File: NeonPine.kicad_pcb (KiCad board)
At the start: 2 copper layers, 54.7 x 69 mm, 102 parts, among them J1 USB-C 16P (USB4105-GF-A), J2 SWD pogo pads, Q1 DMN15H310SE, Q11 MMDT5551, Q12 MMDT5551, Q13 MMDT5551, Q14 MMDT5551, Q15 MMDT5551, Q16 MMDT5551, Q17 MMDT5551, Q18 MMDT5551, Q19 MMDT5551, Q2 TEPT4400, Q20 MMDT5551, U1 CH32V003F4P6, U2 74HC595BQ, U3 74HC595BQ

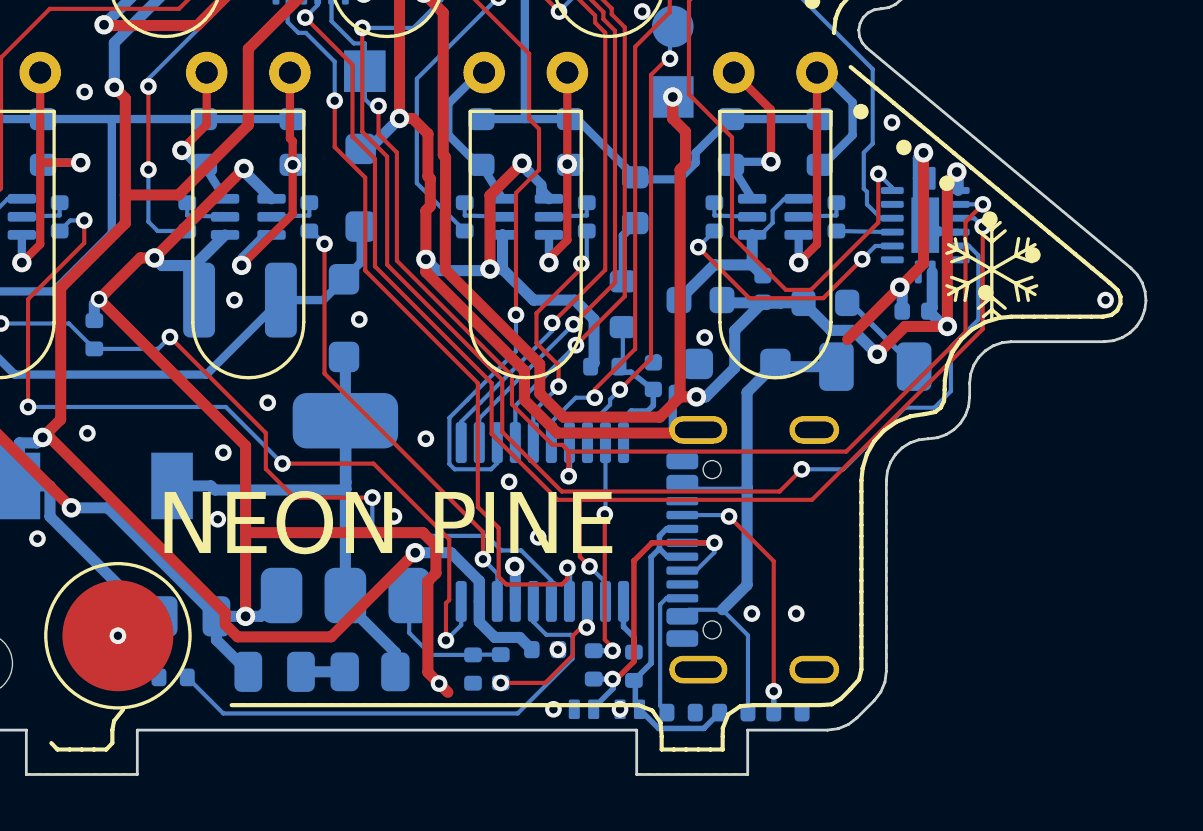
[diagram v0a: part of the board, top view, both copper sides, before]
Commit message: USB clearance fix
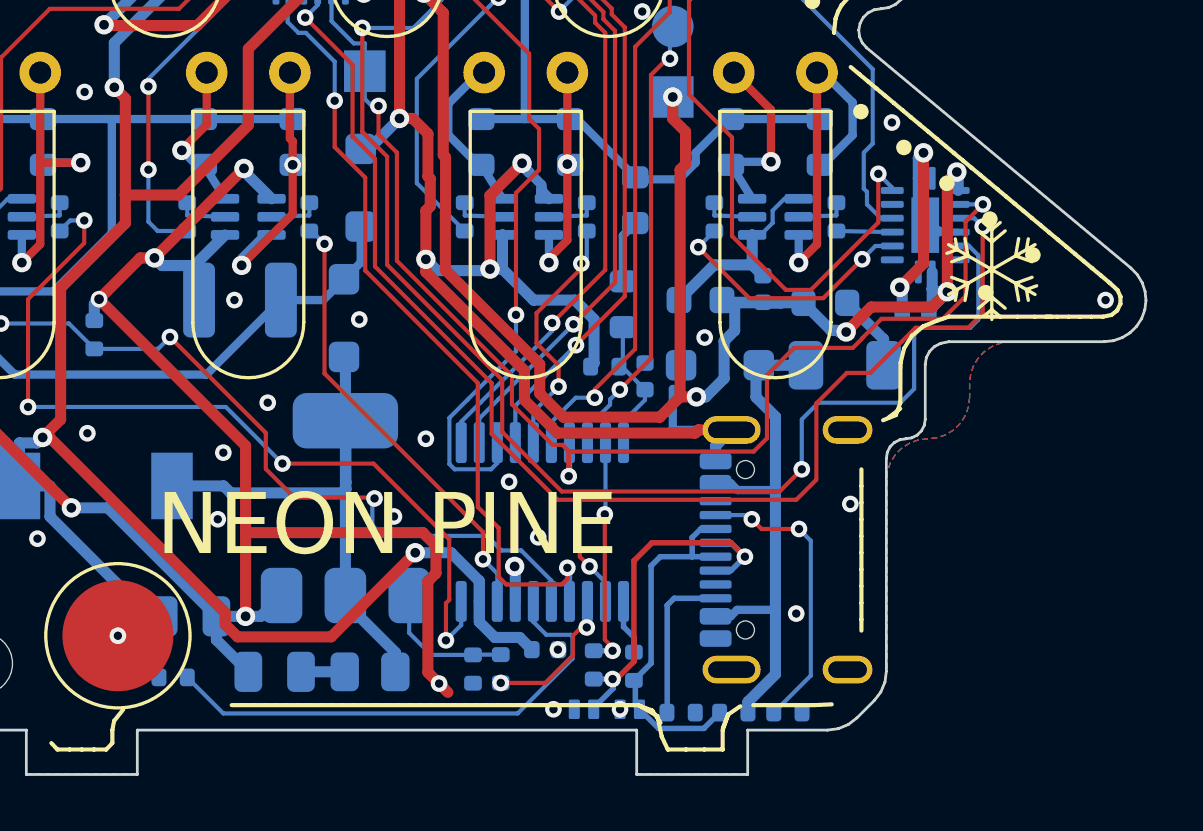
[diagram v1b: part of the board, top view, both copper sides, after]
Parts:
- moved J1 1.20 mm to (115.5, 103.5)
- moved F1 1.10 mm to (116.5, 96.8)
- moved D3 0.60 mm to (112.0, 96.8)
- moved C5 0.30 mm to (109.3, 97.2)
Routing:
- net /SR_LATCH: track 48.8 -> 50.1 mm
- net /SR_CHAIN: track 48.4 -> 49.7 mm
- net /CC1: track 9.44 -> 10.6 mm
- net /USB_DM: track 12.0 -> 13.1 mm
- net /USB_DP: track 12.8 -> 13.7 mm
- net /CC2: track 4.89 -> 5.72 mm
- net /VFB: track 5.74 -> 5.00 mm
- net /SR_CLK: track 45.5 -> 46.1 mm
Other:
- outline, holes or cut-outs redrawn
